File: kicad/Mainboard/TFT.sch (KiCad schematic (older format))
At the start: 2 parts, among them Q1 BSS138

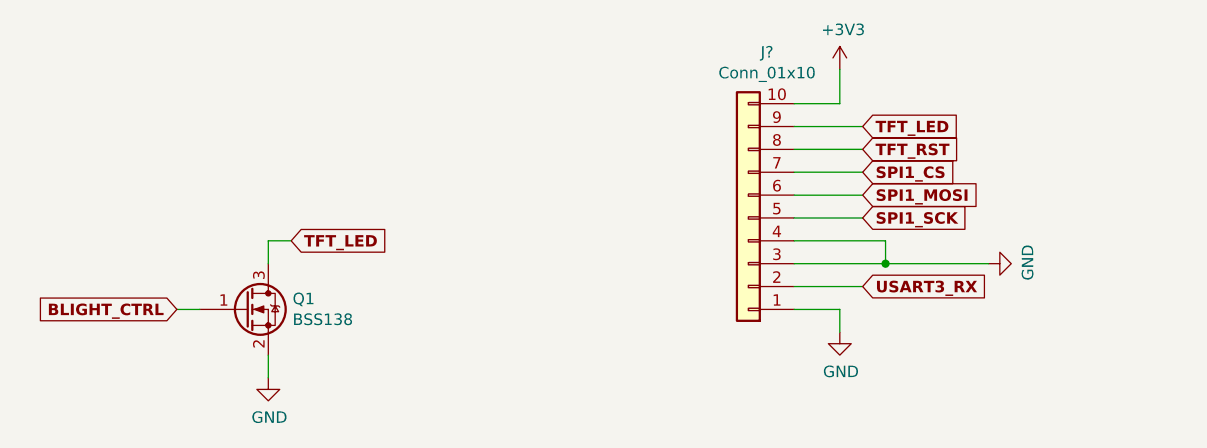
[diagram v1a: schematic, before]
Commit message: Add files via upload
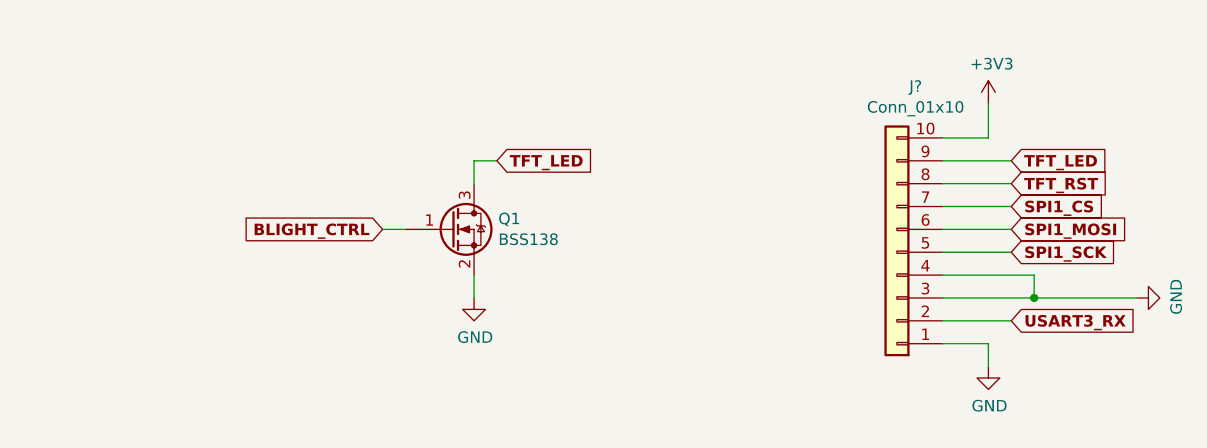
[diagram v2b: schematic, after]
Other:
- moved on the sheet: J?, Q1
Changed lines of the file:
@@
 L Mainboard-rescue:BSS138-transistors Q1
 U 1 1 5DF0AD3D
-P 3400 4100
-F 0 "Q1" H 3606 4146 50  0000 L CNN
-F 1 "BSS138" H 3606 4055 50  0000 L CNN
-F 2 "TO_SOT_Packages_SMD:SOT-23" H 3600 4025 50  0001 L CIN
-F 3 "https://www.fairchildsemi.com/datasheets/BS/BSS138.pdf" H 3400 4100 50  0001 L CNN
-	1    3400 4100
+P 4300 3750
+F 0 "Q1" H 4506 3796 50  0000 L CNN
+F 1 "BSS138" H 4506 3705 50  0000 L CNN
+F 2 "TO_SOT_Packages_SMD:SOT-23" H 4500 3675 50  0001 L CIN
+F 3 "https://www.fairchildsemi.com/datasheets/BS/BSS138.pdf" H 4300 3750 50  0001 L CNN
+	1    4300 3750
 	1    0    0    -1
 $EndComp
@@
 L power:GND #PWR051
 U 1 1 5DF0BBF9
-P 3500 4400
-F 0 "#PWR051" H 3500 4150 50  0001 C CNN
-F 1 "GND" H 3505 4227 50  0000 C CNN
-F 2 "" H 3500 4400 50  0001 C CNN
-F 3 "" H 3500 4400 50  0001 C CNN
-	1    3500 4400
+P 4400 4050
+F 0 "#PWR051" H 4400 3800 50  0001 C CNN
+F 1 "GND" H 4405 3877 50  0000 C CNN
+F 2 "" H 4400 4050 50  0001 C CNN
+F 3 "" H 4400 4050 50  0001 C CNN
+	1    4400 4050
 	1    0    0    -1
 $EndComp
 Wire Wire Line
-	3500 4300 3500 4400
+	4400 3950 4400 4050
 Wire Wire Line
-	3200 4100 3100 4100
-Text GLabel 3100 4100 0    50   Input ~ 10
+	4100 3750 4000 3750
+Text GLabel 4000 3750 0    50   Input ~ 10
 BLIGHT_CTRL
 Wire Wire Line
-	3500 3900 3500 3800
+	4400 3550 4400 3450
 Wire Wire Line
-	3500 3800 3600 3800
-Text GLabel 3600 3800 2    50   Input ~ 10
+	4400 3450 4500 3450
+Text GLabel 4500 3450 2    50   Input ~ 10
 TFT_LED
-Text GLabel 6100 3300 2    50   Input ~ 10
+Text GLabel 6750 3450 2    50   Input ~ 10
 TFT_LED
-Text GLabel 6100 3400 2    50   Input ~ 10
+Text GLabel 6750 3550 2    50   Input ~ 10
 TFT_RST
-Text GLabel 6100 3500 2    50   Input ~ 10
+Text GLabel 6750 3650 2    50   Input ~ 10
 SPI1_CS
-Text GLabel 6100 3600 2    50   Input ~ 10
+Text GLabel 6750 3750 2    50   Input ~ 10
 SPI1_MOSI
-Text GLabel 6100 3700 2    50   Input ~ 10
+Text GLabel 6750 3850 2    50   Input ~ 10
 SPI1_SCK
 Wire Wire Line
-	5800 3300 6100 3300
+	6450 3450 6750 3450
 Wire Wire Line
-	5800 3400 6100 3400
+	6450 3550 6750 3550
 Wire Wire Line
-	5800 3500 6100 3500
+	6450 3650 6750 3650
 Wire Wire Line
-	5800 3600 6100 3600
+	6450 3750 6750 3750
 Wire Wire Line
-	5800 3700 6100 3700
+	6450 3850 6750 3850
 Wire Wire Line
-	5800 3200 6000 3200
+	6450 3350 6650 3350
 Wire Wire Line
-	6000 3200 6000 3050
+	6650 3350 6650 3200
 $Comp
 L power:+3V3 #PWR049
 U 1 1 5DF0DB74
-P 6000 3050
-F 0 "#PWR049" H 6000 2900 50  0001 C CNN
-F 1 "+3V3" H 6015 3223 50  0000 C CNN
-F 2 "" H 6000 3050 50  0001 C CNN
-F 3 "" H 6000 3050 50  0001 C CNN
-	1    6000 3050
+P 6650 3200
+F 0 "#PWR049" H 6650 3050 50  0001 C CNN
+F 1 "+3V3" H 6665 3373 50  0000 C CNN
+F 2 "" H 6650 3200 50  0001 C CNN
+F 3 "" H 6650 3200 50  0001 C CNN
+	1    6650 3200
 	1    0    0    -1
 $EndComp
 Wire Wire Line
-	5800 4100 6000 4100
+	6450 4250 6650 4250
 Wire Wire Line
-	6000 4100 6000 4200
+	6650 4250 6650 4350
 $Comp
 L power:GND #PWR050
 U 1 1 5DF0E0D2
-P 6000 4200
-F 0 "#PWR050" H 6000 3950 50  0001 C CNN
-F 1 "GND" H 6005 4027 50  0000 C CNN
-F 2 "" H 6000 4200 50  0001 C CNN
-F 3 "" H 6000 4200 50  0001 C CNN
-	1    6000 4200
+P 6650 4350
+F 0 "#PWR050" H 6650 4100 50  0001 C CNN
+F 1 "GND" H 6655 4177 50  0000 C CNN
+F 2 "" H 6650 4350 50  0001 C CNN
+F 3 "" H 6650 4350 50  0001 C CNN
+	1    6650 4350
 	1    0    0    -1
 $EndComp
 Wire Wire Line
-	5800 4000 6100 4000
-Text GLabel 6100 4000 2    50   Input ~ 10
+	6450 4150 6750 4150
+Text GLabel 6750 4150 2    50   Input ~ 10
 USART3_RX
 $Comp
 L power:GND #PWR?
 U 1 1 5E1E62B4
-P 6650 3900
-F 0 "#PWR?" H 6650 3650 50  0001 C CNN
-F 1 "GND" H 6655 3727 50  0000 C CNN
-F 2 "" H 6650 3900 50  0001 C CNN
-F 3 "" H 6650 3900 50  0001 C CNN
-	1    6650 3900
+P 7300 4050
+F 0 "#PWR?" H 7300 3800 50  0001 C CNN
+F 1 "GND" H 7305 3877 50  0000 C CNN
+F 2 "" H 7300 4050 50  0001 C CNN
+F 3 "" H 7300 4050 50  0001 C CNN
+	1    7300 4050
 	0    -1   -1   0
 $EndComp
 Wire Wire Line
-	5800 3900 6200 3900
+	6450 4050 6850 4050
 Wire Wire Line
-	5800 3800 6200 3800
+	6450 3950 6850 3950
 Wire Wire Line
-	6200 3800 6200 3900
-Connection ~ 6200 3900
+	6850 3950 6850 4050
+Connection ~ 6850 4050
 Wire Wire Line
-	6200 3900 6650 3900
+	6850 4050 7300 4050
 $Comp
 L Connector_Generic:Conn_01x10 J?
 U 1 1 5E1EAE64
-P 5600 3700
-F 0 "J?" H 5518 2975 50  0000 C CNN
-F 1 "Conn_01x10" H 5518 3066 50  0000 C CNN
-F 2 "" H 5600 3700 50  0001 C CNN
-F 3 "~" H 5600 3700 50  0001 C CNN
-	1    5600 3700
+P 6250 3850
+F 0 "J?" H 6168 3125 50  0000 C CNN
+F 1 "Conn_01x10" H 6168 3216 50  0000 C CNN
+F 2 "" H 6250 3850 50  0001 C CNN
+F 3 "~" H 6250 3850 50  0001 C CNN
+	1    6250 3850
 	-1   0    0    1
 $EndComp
